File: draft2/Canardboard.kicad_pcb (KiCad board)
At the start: 4 copper layers, 63.6 x 50.8 mm, 106 parts, among them IC1 SIC437DED-T1-GE3, J1 RBUS, J2 USB_C_Receptacle_USB2.0, J3 Micro_SD_Card_Det, J4 Conn_01x02_Male, J5 Conn_01x03_Male, J6 Conn_01x03_Male, J7 Conn_01x03_Male, Q1 SI4143DY-T1-GE3, Q2 SI4143DY-T1-GE3, U1 ESP32-S3, U10 LTC4412xS6, U2 SN65HVD230, U3 LM66200DRLR, U5 MAX77827AEFD+T, U6 SC4215, U8 MMC5983MA, U9 LTC4412xS6, Y1 40MHz±10ppm

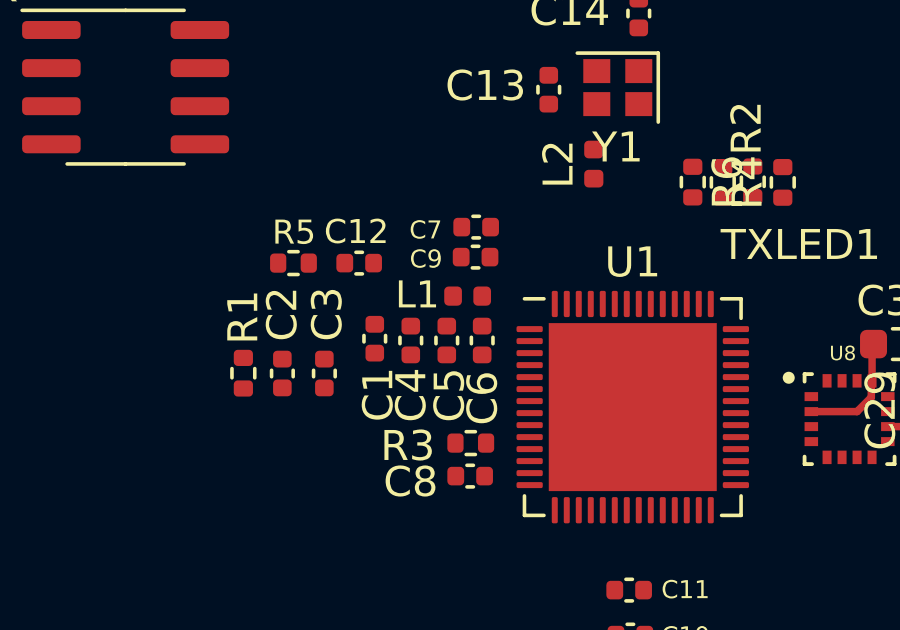
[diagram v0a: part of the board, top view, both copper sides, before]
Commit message: Update Canardboard.kicad_pcb
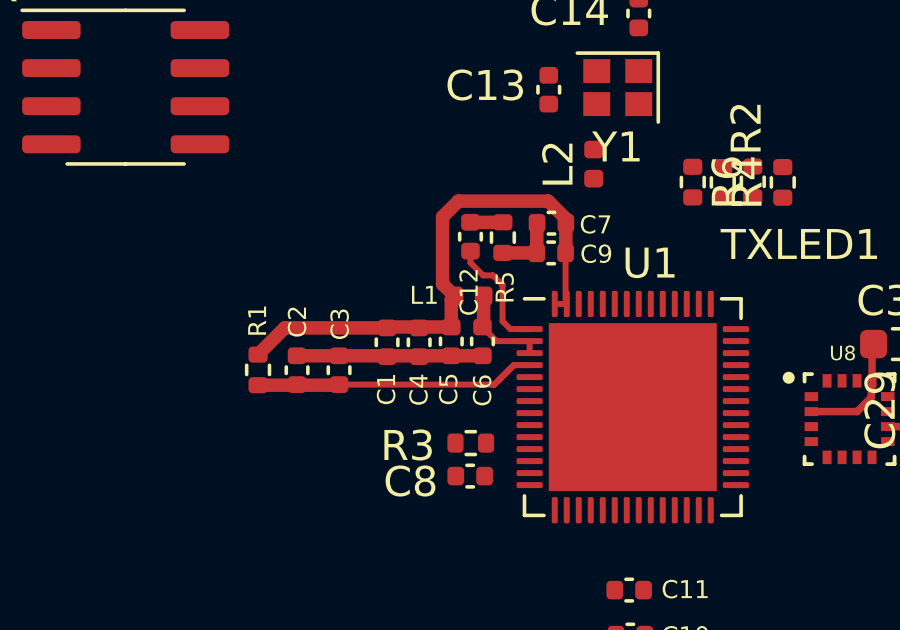
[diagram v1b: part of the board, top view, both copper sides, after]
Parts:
- moved R5 7.03 mm to (132.0, 92.7), turned to 90 degrees
- moved C12 3.81 mm to (130.9, 92.7), turned to -90 degrees
- moved C9 2.52 mm to (133.6, 93.2)
- moved C7 2.51 mm to (133.6, 92.2)
- moved C2 0.50 mm to (125.1, 97.1)
- moved C3 0.50 mm to (126.5, 97.1)
- moved R1 0.50 mm to (123.8, 97.1)
- moved C1 0.43 mm to (128.1, 96.2)
- moved C4 0.29 mm to (129.2, 96.2)
- moved C5 0.15 mm to (130.3, 96.1)
- moved L1 0.05 mm to (130.9, 94.6)
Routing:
- net +3V3: track 9.18 -> 27.7 mm
- net /CHIP_PU: track 0.00 -> 10.3 mm
- net GND: track 56.6 -> 65.0 mm
- net Net-(C12-Pad2): track 0.00 -> 3.99 mm
- net Net-(C6-Pad1): track 0.00 -> 3.21 mm
- net Net-(C12-Pad1): track 0.00 -> 1.08 mm
